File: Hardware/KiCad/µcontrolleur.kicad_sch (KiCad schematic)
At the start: 31 parts, among them J11 Conn_ST_STDC14, SW1 SW_Push, SW3 SW_Push, U1 STM32G431CBUx, Y1 16MHz

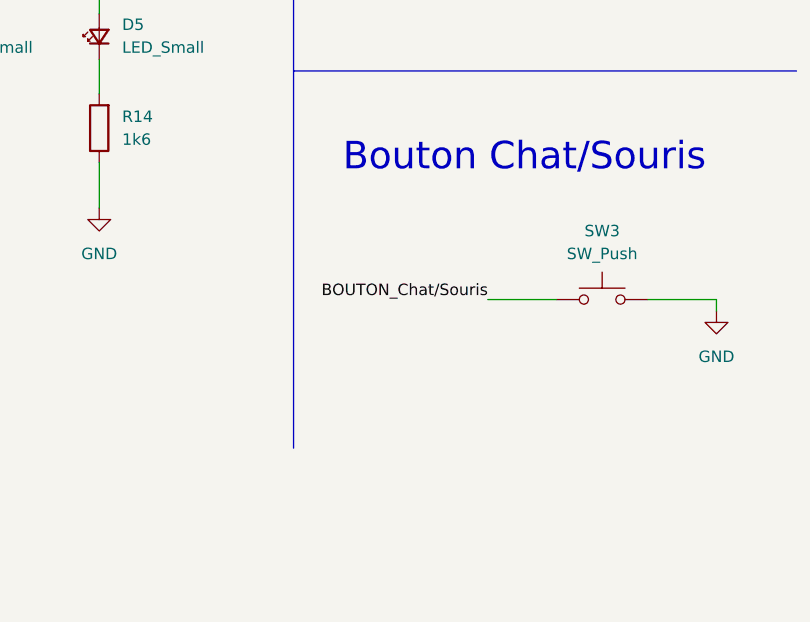
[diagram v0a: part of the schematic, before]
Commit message: s
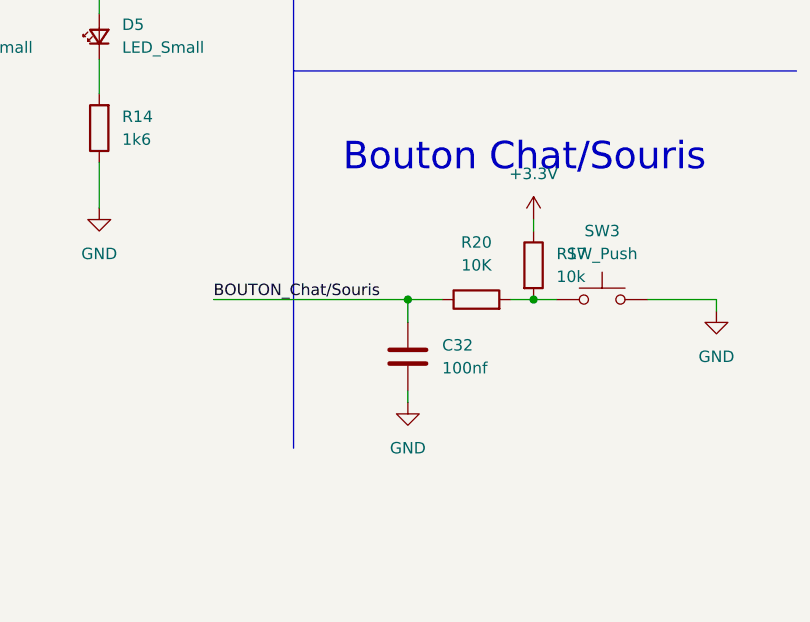
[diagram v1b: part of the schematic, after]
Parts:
- added C32: 100nf, Capacitor_SMD:C_0201_0603Metric, symbol Device:C
- added R17: 10k, Resistor_SMD:R_0603_1608Metric, symbol Device:R
- added R20: 10K, Resistor_SMD:R_0603_1608Metric, symbol Device:R
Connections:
- net +3.3V: now also R17.1
- net BOUTON_Chat/Souris: now also C32.1, R20.1; no longer SW3.1
- net GND: now also C32.2
- new net: R17.2, R20.2, SW3.1
